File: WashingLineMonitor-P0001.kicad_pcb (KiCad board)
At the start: 2 copper layers, 58.5 x 43.5 mm, 73 parts, among them J1 S1711-46R, J2 S1711-46R, J3 Conn_02x03_Odd_Even, Q1 PJA3401A_R1_00001, Q3 Q_Dual_NMOS_PMOS_G1S2G2D2S1D1, SW1 A6TN-1104, U1 HDC2080, U2 TLV2371DBV, U3 ESP32-C6-MINI-1, U5 TLV75533PDBV, U6 BQ51050BRHL

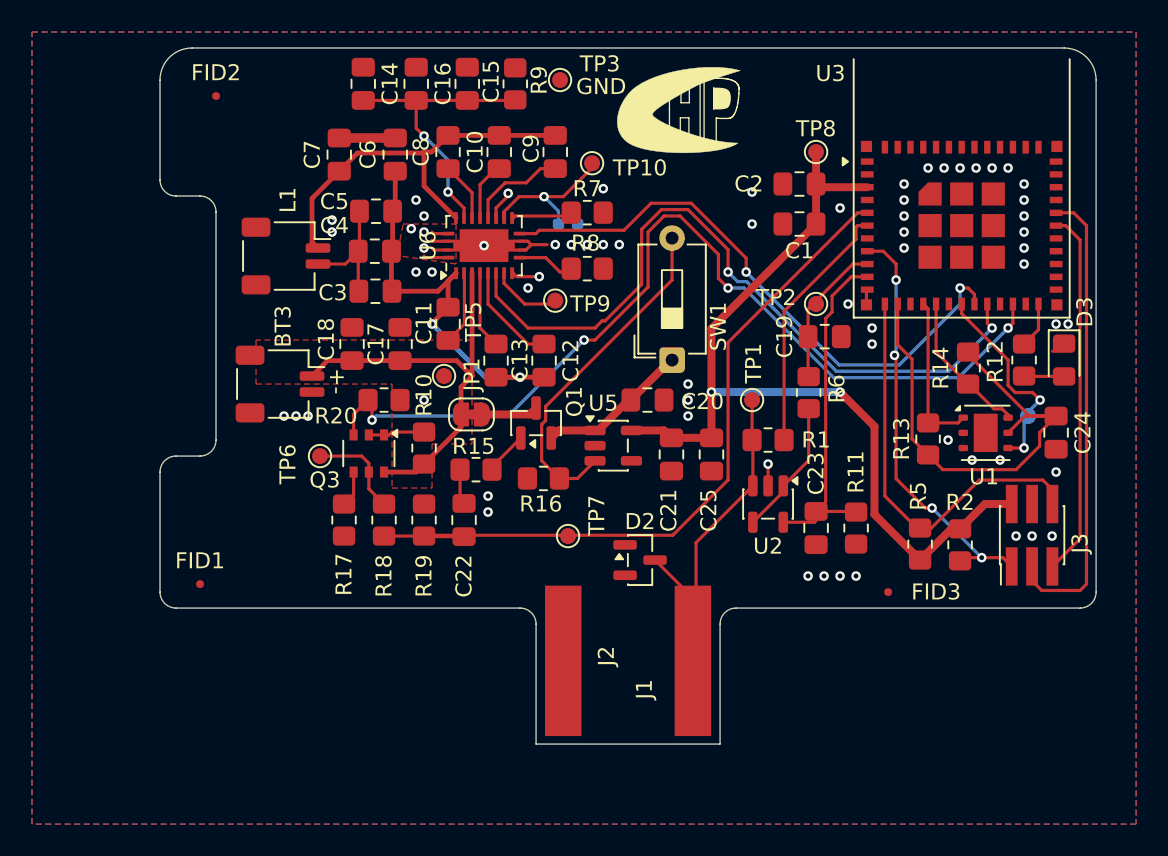
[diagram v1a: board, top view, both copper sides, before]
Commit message: finished board layout for AD revision
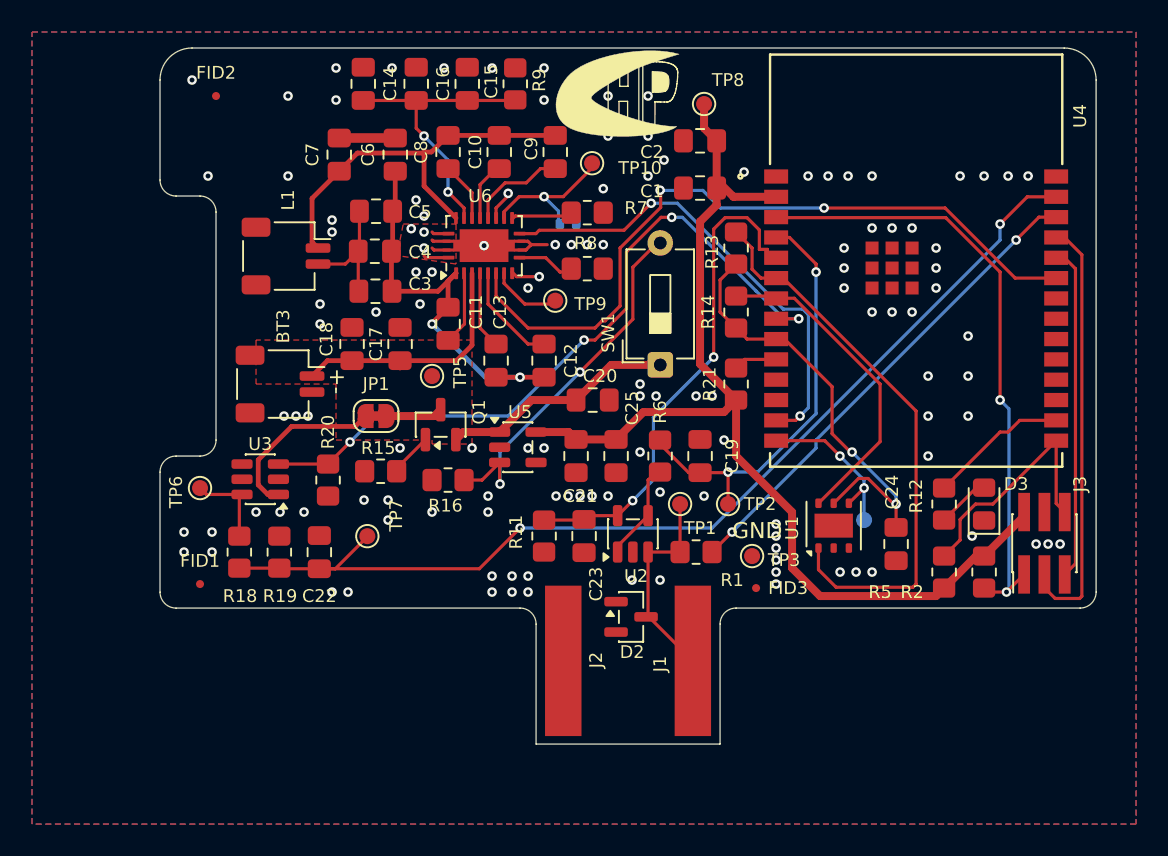
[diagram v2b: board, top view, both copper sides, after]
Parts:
- removed Q3: Q_Dual_NMOS_PMOS_G1S2G2D2S1D1, Package_SO:TSOP-6_1.65x3.05mm_P0.95mm
- removed R10: 500k, Resistor_SMD:R_0805_2012Metric_Pad1.20x1.40mm_HandSolder
- removed R17: 10k, Resistor_SMD:R_0805_2012Metric_Pad1.20x1.40mm_HandSolder
- added R21: 10k, Resistor_SMD:R_0805_2012Metric_Pad1.20x1.40mm_HandSolder, F.Cu at (153.0, 93.0)
- added U4: ESP32-C6-WROOM-1-N4, Hydro_footprints:MOD28_ESP32-C6-WROOM-1_EXP, F.Cu at (164.3, 85.3)
- TH1: footprint Resistor_SMD:R_0402_1005Metric_Pad0.72x0.64mm_HandSolder -> Resistor_SMD:R_0402_1005Metric
- U3: value ESP32-C6-MINI-1 -> TPS22810DBV; footprint RF_Module:ESP32-C6-MINI-1 -> Package_TO_SOT_SMD:SOT-23-6
- moved U3 46.6 mm to (123.3, 99.0), turned to 180 degrees
- moved TP3 32.1 mm to (154.0, 103.8)
- moved R11 19.5 mm to (141.0, 102.5)
- moved R13 16.9 mm to (153.0, 84.5)
- moved R14 14.9 mm to (153.0, 88.5), turned to 90 degrees
- moved C23 14.5 mm to (143.5, 102.5)
- moved TP2 13.7 mm to (152.5, 100.5)
- moved TP7 12.5 mm to (130.0, 102.5)
- moved C24 12.2 mm to (163.0, 103.0)
- moved TP4 12.1 mm to (161.0, 101.5)
- moved U1 11.1 mm to (159.1, 101.8), turned to 90 degrees
- moved C19 10.8 mm to (150.8, 97.5), turned to 90 degrees
- moved D3 10.3 mm to (168.5, 100.5), turned to 90 degrees
- moved R12 10.3 mm to (166.0, 100.5)
- moved R6 10.1 mm to (148.2, 97.5)
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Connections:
- R12 pad 1: Net-(U3-IO18) -> Net-(U4-IO18)
- R18 pad 1: Net-(Q3A-S) -> Net-(U3-VOUT)
- TP6 pad 1: Net-(Q3A-S) -> Net-(U3-VOUT)
- U3 pad 1: GND -> Vbatt
- U3 pad 3: 3V3 -> MEAS_BATT
- U3 pad 5: Battery_Voltage -> unconnected-(U3-QOD-Pad5)
- U3 pad 6: SENSOR_PWR -> Net-(U3-VOUT)
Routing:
- net SDA: track 9.89 -> 35.5 mm
- net Battery_Voltage: track 46.1 -> 65.2 mm, vias 0 -> 2
- net SENSOR_OUTPUT: track 9.11 -> 26.9 mm, vias 0 -> 2
- net SENSOR_PWR: track 15.9 -> 30.5 mm, vias 0 -> 2
- net MEAS_BATT: track 58.9 -> 44.6 mm
- net ESP_EN: track 26.6 -> 38.7 mm, vias 4 -> 2
- net 3V3: track 56.8 -> 68.0 mm, vias 2 -> 0
- net SCL: track 9.33 -> 20.3 mm
- net OP_AMP_POWER: track 21.2 -> 31.8 mm, vias 0 -> 2
- net ESP_BOOT: track 25.7 -> 15.4 mm
- net Net-(U4-IO18): track 0.00 -> 8.76 mm
- net /Moisture Sensor/Vsens: track 20.6 -> 13.0 mm
- net QI_EN2: track 37.3 -> 29.9 mm
- net Net-(Q3A-S): track 6.18 -> 0.00 mm
- net Net-(U3-VOUT): track 0.00 -> 5.47 mm
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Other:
- board text added: "HoratioPistachio WashingLineMonitor-P0001_AD"
- board text removed: "HoratioPistachio WashingLineMonitor-P0001_AC"
